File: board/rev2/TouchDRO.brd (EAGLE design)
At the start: 50.8 x 50.8 mm, 29 parts, among them U2 VREG_33, U3 VREG_5

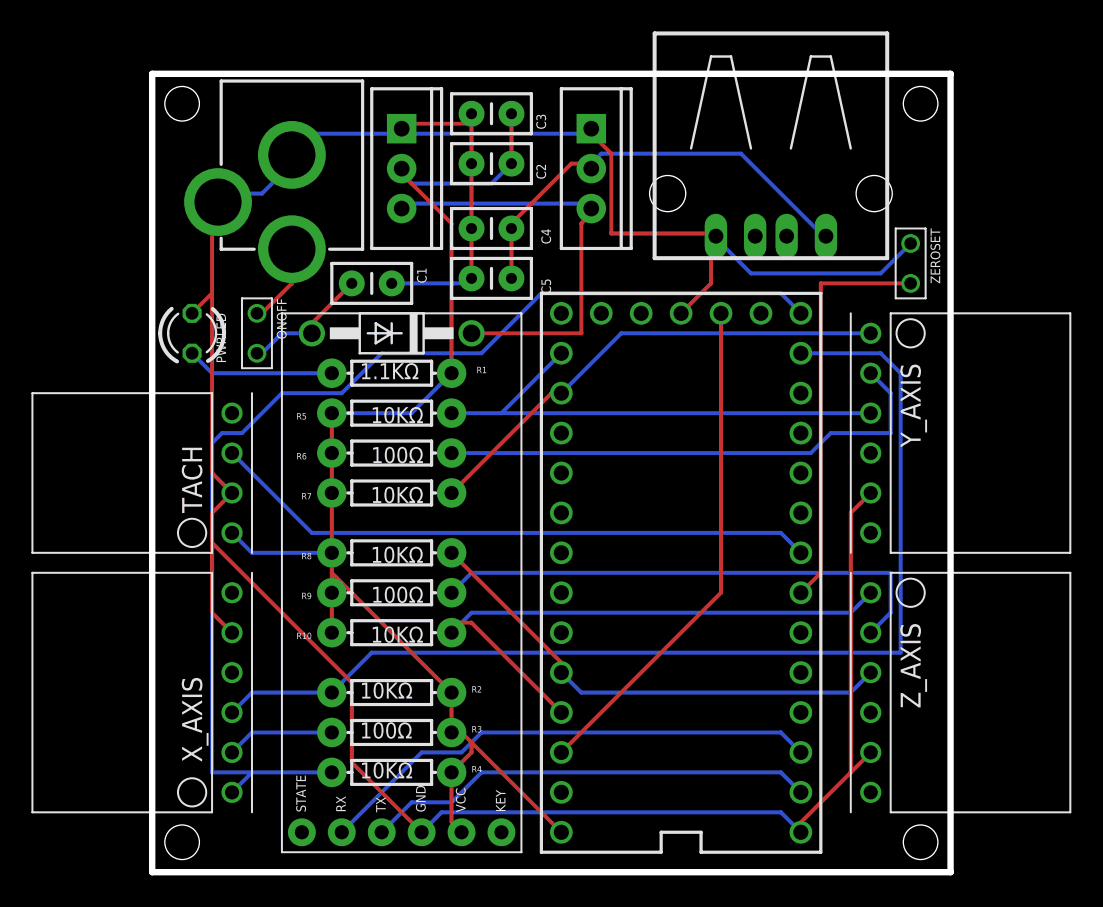
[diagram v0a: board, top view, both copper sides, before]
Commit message: cleaned up connector components. updated images
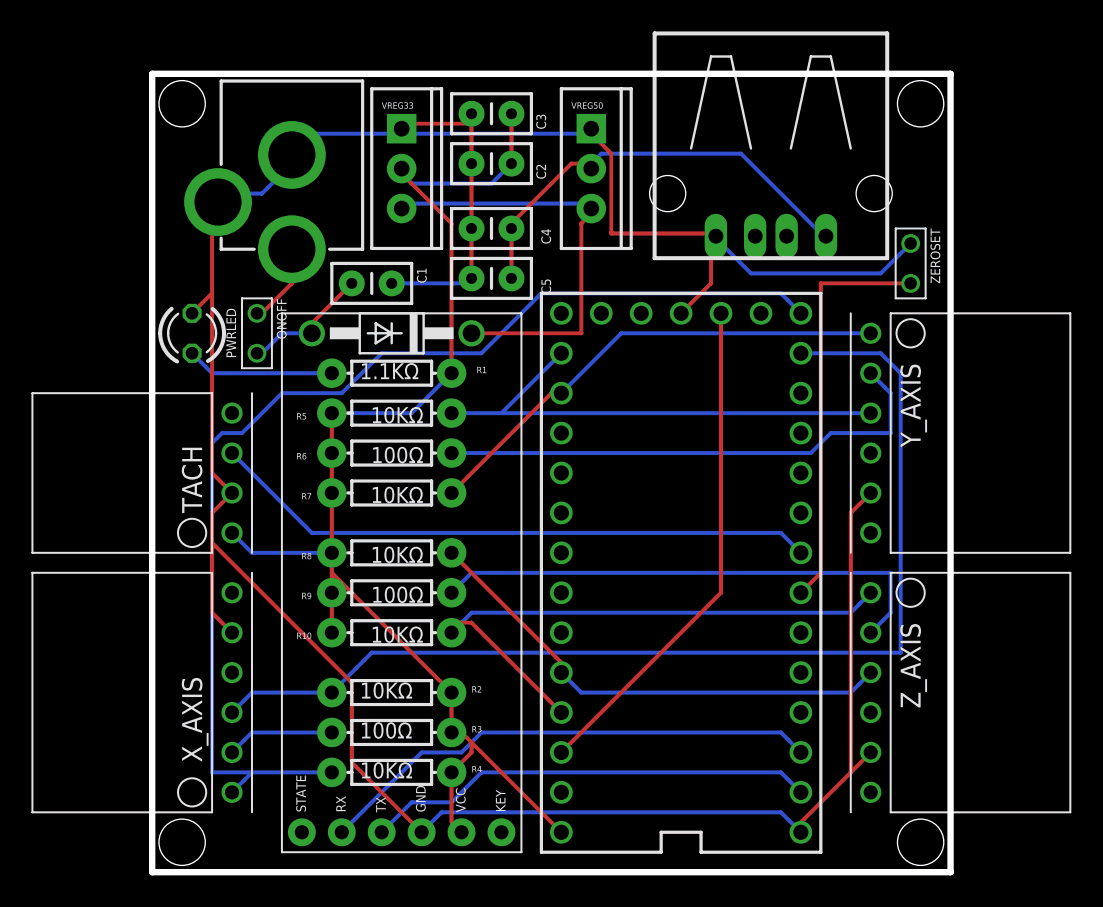
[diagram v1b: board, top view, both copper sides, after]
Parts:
- renumbered U2 to VREG33, U3 to VREG50
